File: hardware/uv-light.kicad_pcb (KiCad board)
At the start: 2 copper layers, 25 x 15 mm, 18 parts, among them P1 CON-SENSOR, U1 M24C64, U2 VEML6070, U3 DRILL, U4 DRILL, U5 DRILL, U6 DRILL

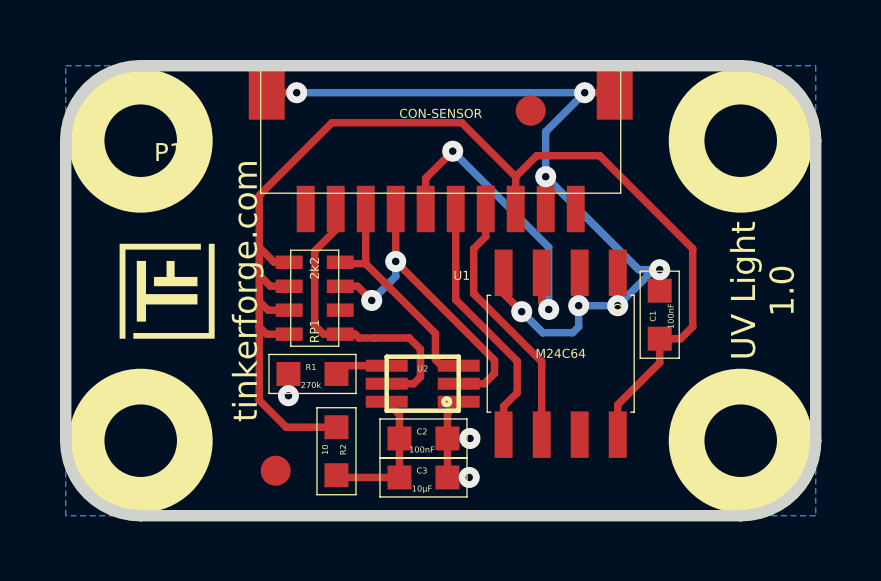
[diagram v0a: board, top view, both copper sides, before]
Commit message: Add 3d information (final)
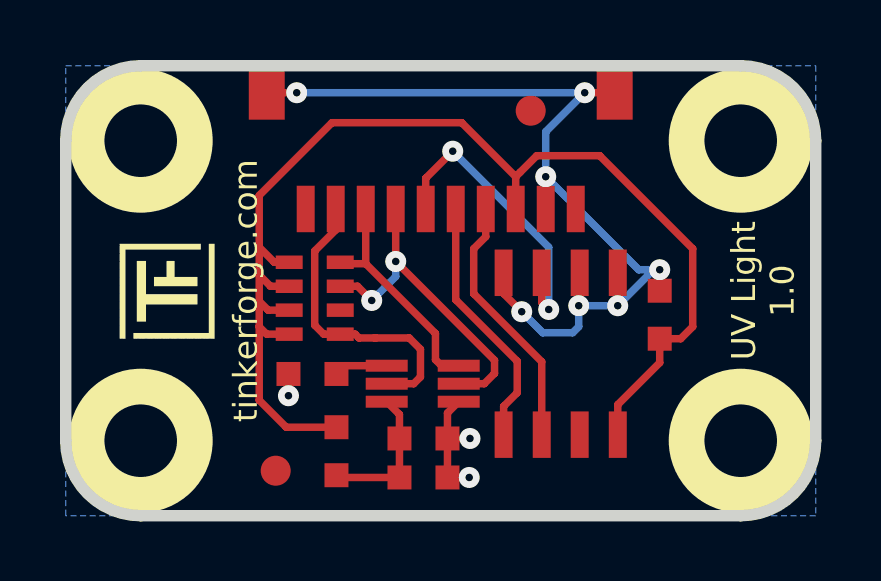
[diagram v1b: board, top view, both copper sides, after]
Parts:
- C1, C2, C3: footprint kicad-libraries:0603 -> kicad-libraries:C0603
- R1, R2: footprint kicad-libraries:0603 -> kicad-libraries:R0603
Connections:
- P1 pad 1: (no net) -> Net-(P1-Pad1)
- P1 pad 10: (no net) -> Net-(P1-Pad10)
- RP1 pad 6: (no net) -> Net-(RP1-Pad6)
- U1 pad 7: (no net) -> Net-(U1-Pad7)
